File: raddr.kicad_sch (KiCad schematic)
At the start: 8 parts, among them J1 Conn_01x01, J2 Conn_01x01, J3 Conn_01x03, J4 Conn_01x04, U1 PMS150C-U06

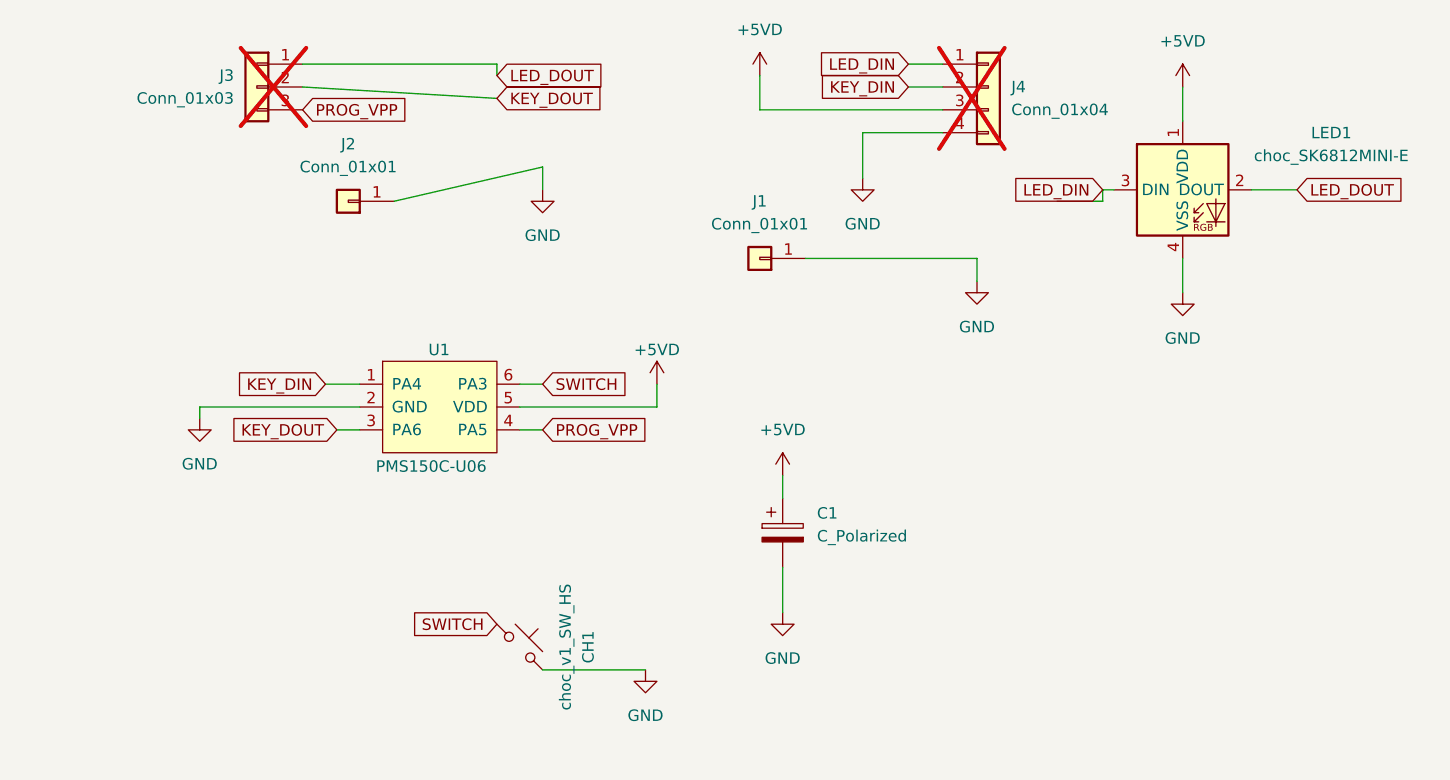
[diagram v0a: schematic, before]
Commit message: Silk screen adjustments.
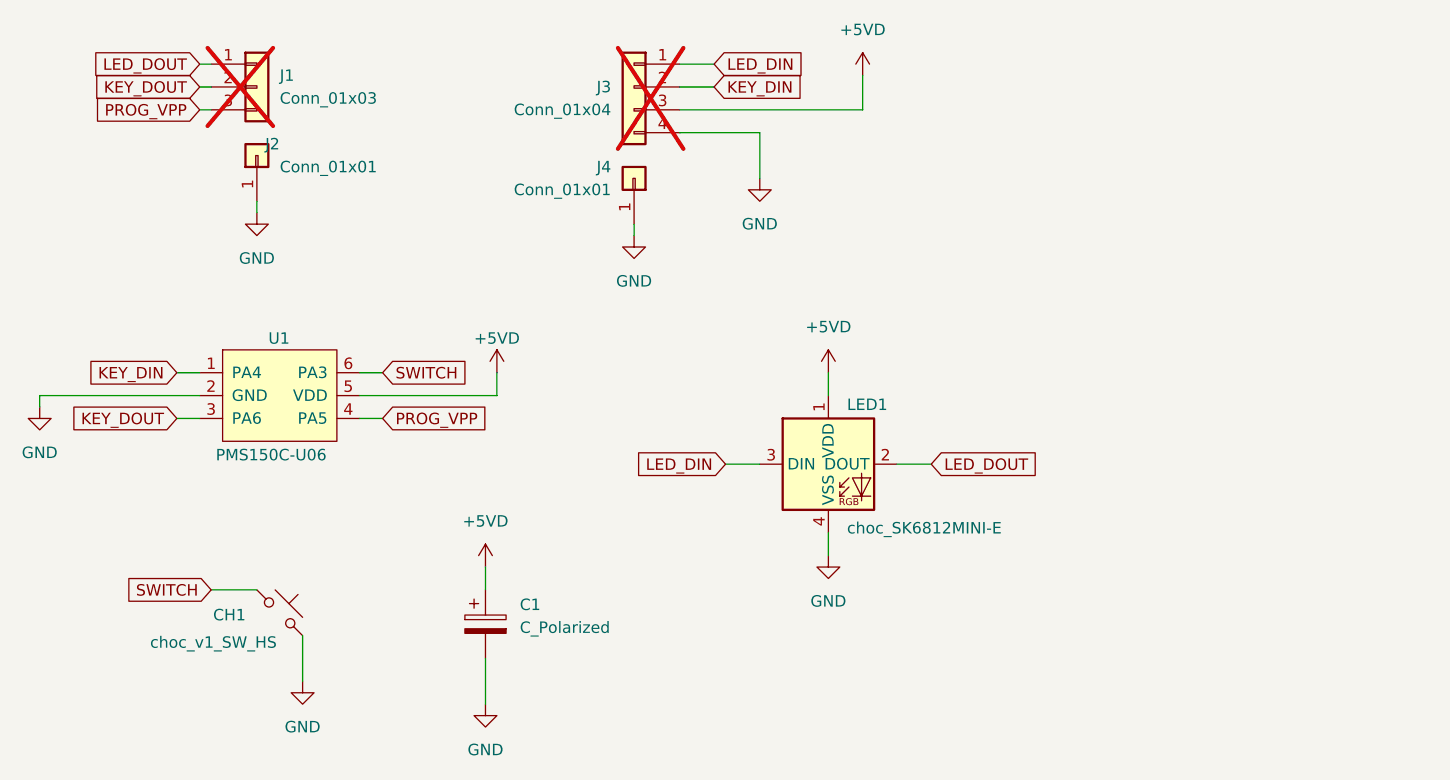
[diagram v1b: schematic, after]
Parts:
- renumbered J3 to J1, J4 to J3, J1 to J4
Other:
- moved on the sheet: C1, CH1, J1, J2, J3, J4, LED1, U1
